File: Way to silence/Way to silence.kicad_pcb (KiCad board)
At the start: 2 copper layers, 62 parts, among them J1 SD Card Connector, J2 Amplificator_Terminal, J3 5V_Terminal, J4 Battery_Terminal, Q1 BC817, Q2 BC817, SW1 SW_SPDT, U1 ESP32-WROOM-32-N16, U2 SM5308, U3 CP2102-GMR, U4 MAX98357AETE+T, U5 USB-TYPE-C-018, U6 AMS1117CD-3.3

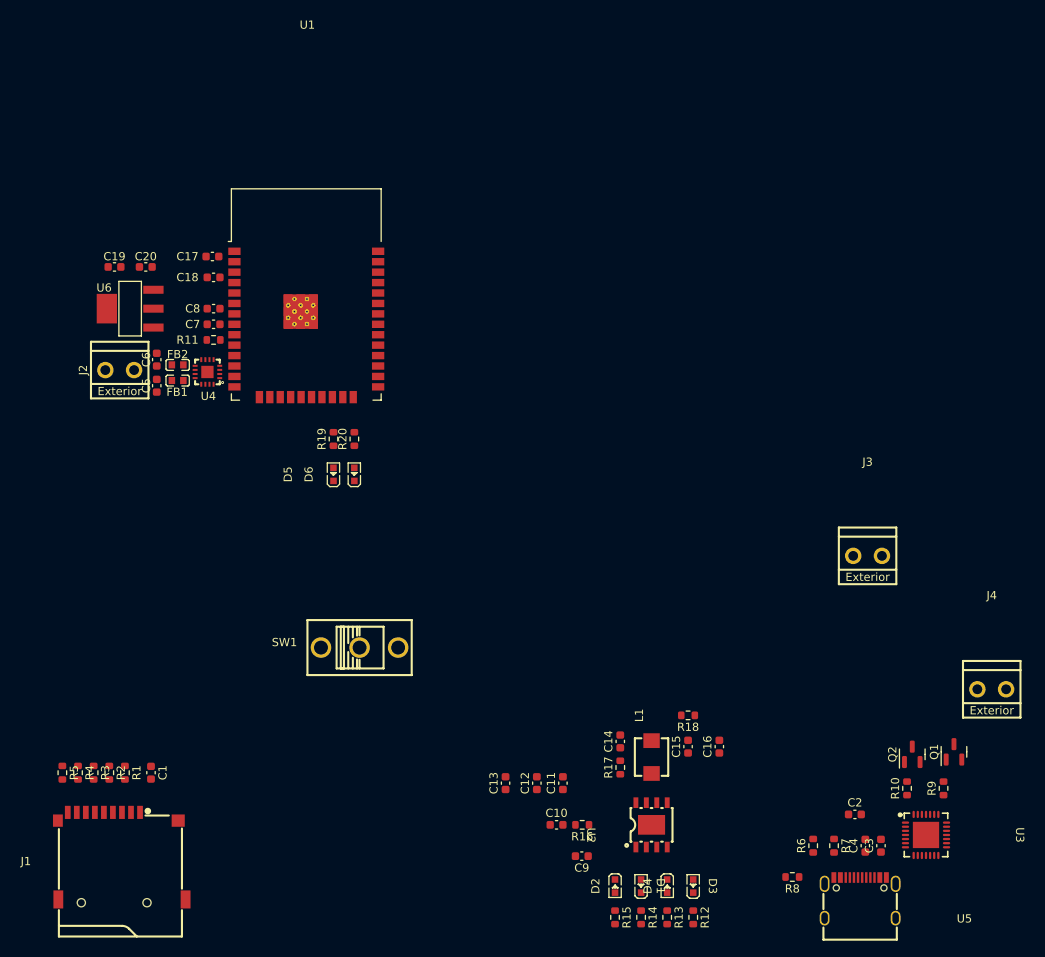
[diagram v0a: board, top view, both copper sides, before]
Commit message: [ADD] Routing placement seems ok
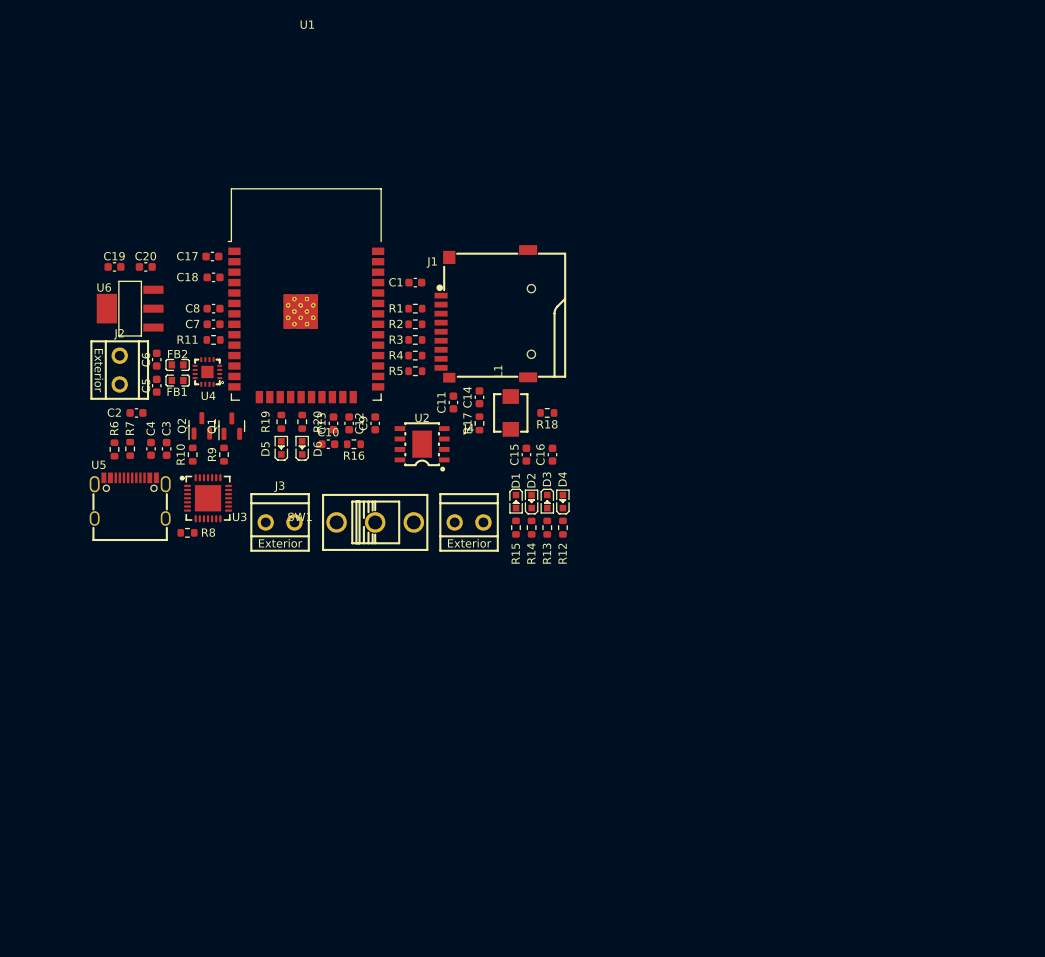
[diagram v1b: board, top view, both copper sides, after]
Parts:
- moved U5 101.4 mm to (68.6, 75.8)
- moved C2 100.2 mm to (69.4, 65.4)
- moved C3 99.5 mm to (73.0, 69.8)
- moved C4 99.5 mm to (71.1, 69.8)
- moved R7 98.4 mm to (68.6, 69.8)
- moved R6 97.8 mm to (66.7, 69.8)
- moved R9 96.6 mm to (80.0, 70.5)
- moved U3 96.6 mm to (78.1, 75.8)
- moved Q1 96.5 mm to (81.0, 67.0)
- moved R10 96.0 mm to (76.2, 70.5)
- moved Q2 95.3 mm to (77.3, 67.0)
- moved R8 84.7 mm to (75.6, 80.0), turned to 0 degrees
- moved J1 79.4 mm to (111.7, 53.3), turned to 90 degrees
- moved J3 71.7 mm to (86.8, 78.7)
- moved C1 67.8 mm to (103.3, 49.5), turned to 0 degrees
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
